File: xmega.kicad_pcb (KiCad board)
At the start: 2 copper layers, 96.5 x 50.8 mm, 93 parts, among them IC1 ATXMEGA128A3U-A, P1 PH_PWR, P3 PH_CURRENT, P5 USB_OTG, P6 PH_TWI, P7 PH_PA, P8 CONN_01X16, Q1 SI2323DS, SW0 TACTB-24R-F, SW1 TACTB-24R-F, SW2 TACTB-24R-F, SW3 TACTB-24R-F, U1 AT45DB161E - EIAJ SOIC, U2 MC78M05CDT, U3 AP1117, U4 LM4040BIM3-2.5, U5 USBLC62, U6 MAX3232EID, U7 micro_sd_card

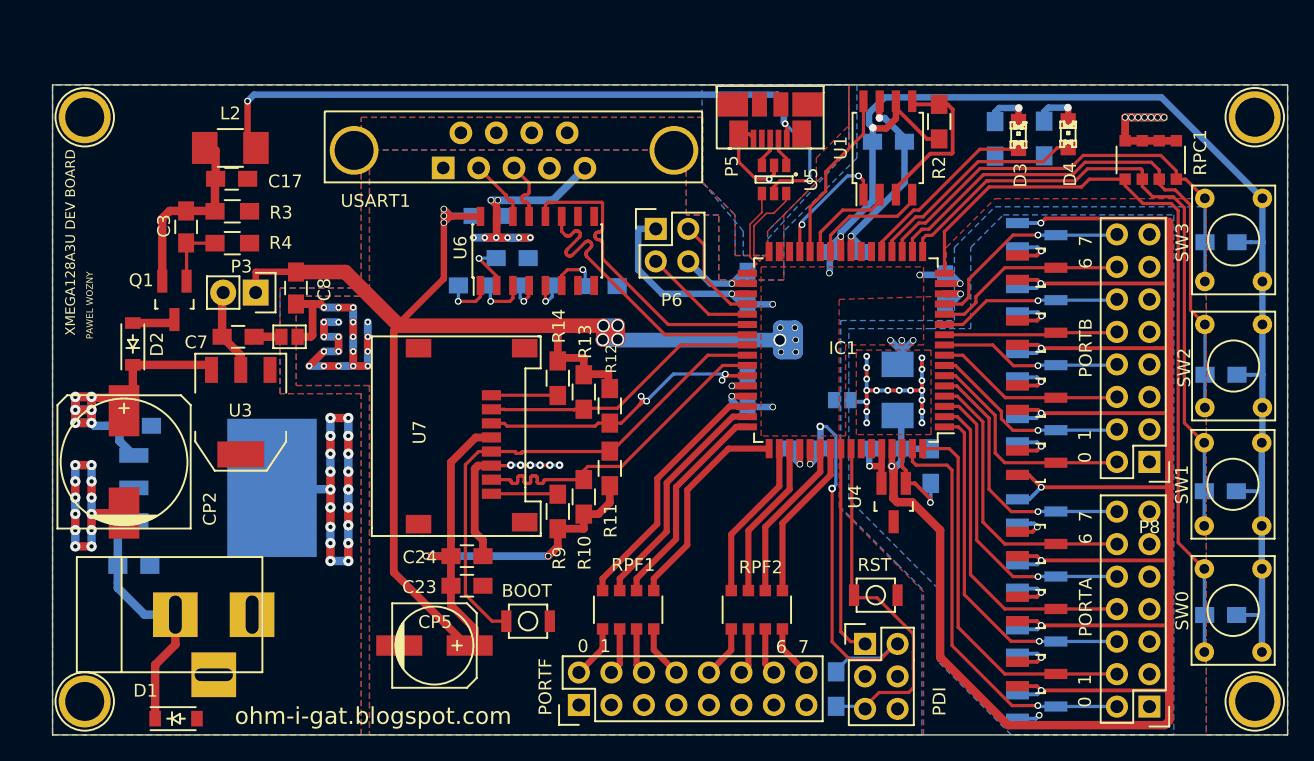
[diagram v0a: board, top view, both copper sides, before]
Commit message: dd
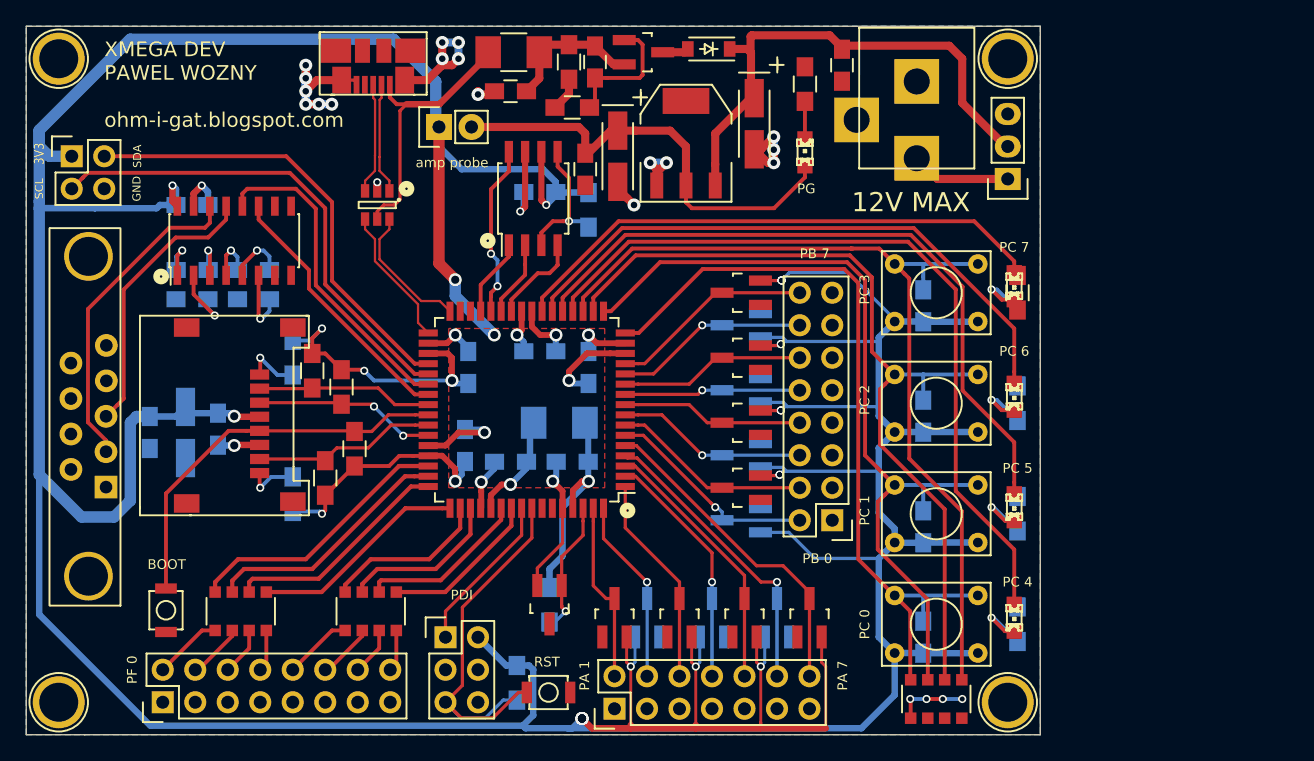
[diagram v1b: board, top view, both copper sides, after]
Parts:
- removed BOOT: boot, woznyLIB:B3U-1000P
- removed C24: 1n, Capacitors_SMD:C_0805_HandSoldering
- removed C25, C26, C27, C28, C4: 100n, Capacitors_SMD:C_0805_HandSoldering
- removed CP2: 100u, Capacitors_SMD:c_elec_10x7.7
- removed CP5: 100u, Capacitors_SMD:c_elec_6.3x5.3
- removed D1: SS14, Diodes_SMD:SOD-123
- removed Digital: PH_DIGITAL IO, Pin_Headers:Pin_Header_Straight_2x08
- removed JP1, JP2: Jumper_NC_Small, Connect:GS2
- removed PDI: PH_PDI, Pin_Headers:Pin_Header_Straight_2x03
- removed R5: 17k8, Resistors_SMD:R_0805_HandSoldering
- removed the REF** at (58.4, 119.3)
- removed the REF** at (58.4, 73.6)
- removed the REF** at (149.8, 119.3)
- removed the REF** at (149.8, 73.6)
- removed RST: rst, woznyLIB:B3U-1000P
- removed SW0: TACTB-24R-F, woznyLIB:B3F-1022
- removed U7: micro_sd_card, woznyLIB:112C-TBAR-R02
- added C19: 100n, Capacitors_SMD:C_0805_HandSoldering, B.Cu at (66.8, 85.6)
- added C20: 100n, Capacitors_SMD:C_0805_HandSoldering, B.Cu at (71.6, 85.6)
- added C21: 100n, Capacitors_SMD:C_0805_HandSoldering, B.Cu at (66.8, 80.5)
- added C22: 100n, Capacitors_SMD:C_0805_HandSoldering, B.Cu at (66.8, 87.9)
- added CT1: 100u, Capacitors_Tantalum_SMD:TantalC_SizeA_EIA-3216_HandSoldering, F.Cu at (110.7, 74.2)
- added CT2: 100u, Capacitors_Tantalum_SMD:TantalC_SizeA_EIA-3216_HandSoldering, F.Cu at (100.1, 76.7)
- added CT3: 100u, Capacitors_Tantalum_SMD:TantalC_SizeA_EIA-3216_HandSoldering, B.Cu at (66.3, 98.3)
- added D21: LED, LEDs:LED-0805, F.Cu at (131.0, 104.1)
- added D22: LED, LEDs:LED-0805, F.Cu at (131.0, 112.8)
- added D5: Dprot, Housings_SOT-23_SOT-143_TSOT-6:SOT-23_Handsoldering, B.Cu at (102.4, 112.8)
- added P2: PH_PDI, Pin_Headers:Pin_Header_Straight_2x03, F.Cu at (86.6, 114.3)
- added P4: PH_DIGITAL IO, Pin_Headers:Pin_Header_Straight_2x08, F.Cu at (64.5, 119.4)
- added R16: 220, Resistors_SMD:R_0805_HandSoldering, B.Cu at (131.3, 104.6)
- added R17: 220, Resistors_SMD:R_0805_HandSoldering, B.Cu at (131.3, 113.3)
- added R6: 220, Resistors_SMD:R_0805_HandSoldering, F.Cu at (114.7, 71.1)
- added R7: 17k8, Resistors_SMD:R_0805_HandSoldering, B.Cu at (94.7, 111.7)
- added REF**: 1pin, Connect:1pin, F.Cu at (56.4, 69.1)
- added REF**: 1pin, Connect:1pin, F.Cu at (130.5, 69.1)
- added REF**: 1pin, Connect:1pin, F.Cu at (56.4, 119.4)
- added REF**: 1pin, Connect:1pin, F.Cu at (130.5, 119.4)
- added SW4: TACTB-24R-F, woznyLIB:SWITCH__B3F-1022, F.Cu at (124.9, 113.3)
- added SW5: TACTB-24R-F, woznyLIB:SWITCH__B3F-1022, F.Cu at (124.9, 104.6)
- added SW6: TACTB-24R-F, woznyLIB:SWITCH__B3F-1022, F.Cu at (124.9, 96.0)
- added SW7: TACTB-24R-F, woznyLIB:SWITCH__B3F-1022, F.Cu at (124.9, 87.4)
- C1, C12, C2, D10, D12, D14, D16, D18, D6, D8: moved to F.Cu
- C14: value 100n -> 1n
- C17, C23, C7, C8, D11, D13, D15, D17, D7, D9, R13, R2: moved to B.Cu
- D19: value Dprot -> LED; footprint Housings_SOT-23_SOT-143_TSOT-6:SOT-23_Handsoldering -> LEDs:LED-0805
- D20: value Dprot -> LED; footprint Housings_SOT-23_SOT-143_TSOT-6:SOT-23_Handsoldering -> LEDs:LED-0805; moved to F.Cu
- D3: value LED -> PG3.3
- D4: value LED -> Dprot; footprint LEDs:LED-0805 -> Housings_SOT-23_SOT-143_TSOT-6:SOT-23_Handsoldering
- P1: footprint Connect:BARREL_JACK -> woznyLIB:BARREL_JACK
- P5: footprint woznyLIB:G3515-10 -> woznyLIB:uUSB__G3515-10
- P6: value PH_TWI -> PH_PA; footprint Pin_Headers:Pin_Header_Straight_2x02 -> Pin_Headers:Pin_Header_Straight_2x07
- P7: value PH_PA -> CONN_01X16; footprint Pin_Headers:Pin_Header_Straight_2x07 -> Pin_Headers:Pin_Header_Straight_2x08
- P8: value CONN_01X16 -> PH_TWI; footprint Pin_Headers:Pin_Header_Straight_2x08 -> Pin_Headers:Pin_Header_Straight_2x02
- R14: value 50K -> 220
- R8: value 220 -> 50K
- SW1: value TACTB-24R-F -> boot; footprint woznyLIB:B3F-1022 -> woznyLIB:SWITCH__B3U-1000P
- SW2: value TACTB-24R-F -> rst; footprint woznyLIB:B3F-1022 -> woznyLIB:SWITCH__B3U-1000P
- SW3: value TACTB-24R-F -> SPST; footprint woznyLIB:B3F-1022 -> Pin_Headers:Pin_Header_Straight_1x03
- U2: value MC78M05CDT -> AP1117; footprint SMD_Packages:TO-263 -> SMD_Packages:SOT-223; moved to F.Cu
- U3: value AP1117 -> LM4040BIM3-2.5; footprint SMD_Packages:SOT-223 -> Housings_SOT-23_SOT-143_TSOT-6:SOT-23_Handsoldering
- U4: value LM4040BIM3-2.5 -> USBLC62; footprint Housings_SOT-23_SOT-143_TSOT-6:SOT-23_Handsoldering -> Housings_SOT-23_SOT-143_TSOT-6:SOT-23-6
- U5: value USBLC62 -> micro_sd_card; footprint Housings_SOT-23_SOT-143_TSOT-6:SOT-23-6 -> woznyLIB:SDcard__112C-TBAR-R02
- USART1: footprint woznyLIB:DBR09F -> woznyLIB:USART__DBR09F
- moved P8 87.5 mm to (57.4, 76.7), turned to 0 degrees
- moved SW1 84.2 mm to (64.7, 113.9), turned to 90 degrees
- moved P1 71.6 mm to (123.4, 70.7), turned to 270 degrees
- moved R8 61.5 mm to (74.7, 103.1), turned to 90 degrees
- moved SW2 57.8 mm to (96.3, 118.6), turned to 180 degrees
- moved C17 57.1 mm to (123.9, 97.0), turned to 90 degrees
- moved C13 56.2 mm to (63.5, 98.3), turned to 270 degrees
- moved D4 51.8 mm to (99.8, 112.8), turned to 0 degrees
- moved U2 50.9 mm to (105.4, 75.7), turned to 0 degrees
- moved D2 50.6 mm to (107.2, 68.3), turned to 180 degrees
- moved U5 46.8 mm to (69.1, 96.5)
- moved U4 46.6 mm to (81.3, 80.5), turned to 270 degrees
- moved C14 45.9 mm to (68.8, 98.0), turned to 270 degrees
- moved RPC1 45.3 mm to (124.9, 119.1)
- moved Q1 41.5 mm to (102.1, 68.6), turned to 270 degrees
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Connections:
- C1 pad 1: Net-(C1-Pad1) -> +5V
- C10 pad 2: GNDD -> GND
- C11 pad 1: +3V3 -> +3.3VADC
- C11 pad 2: GNDD -> GND
- C12 pad 1: +3V3 -> +5V
- C12 pad 2: GNDD -> GND
- C13 pad 2: GNDD -> GND
- C14 pad 2: GNDD -> GND
- C15 pad 2: GNDD -> /buttons/O0
- C16 pad 1: +3.3VADC -> +3V3
- C16 pad 2: GNDA -> /buttons/O1
- C17 pad 1: +5V -> +3V3
- C17 pad 2: GND -> /buttons/O2
- C18 pad 1: GNDD -> +3V3
- C18 pad 2: Net-(C18-Pad2) -> /buttons/O3
- C2 pad 2: Net-(C2-Pad2) -> GND
- C23 pad 1: +3V3 -> GND
- C23 pad 2: GNDD -> Net-(C23-Pad2)
- C3 pad 1: +5V -> /Vcc_5_3V/CC0
- C3 pad 2: Net-(C3-Pad2) -> GND
- C5 pad 1: /Vcc_5_3V/5VUSB -> +3V3
- C6 pad 1: GNDD -> +3V3
- C6 pad 2: +3V3 -> GND
- C7 pad 1: /Vcc_5_3V/CC0 -> +3V3
- C8 pad 2: GNDD -> GND
- C9 pad 1: GNDD -> +3V3
- C9 pad 2: Net-(C9-Pad2) -> GND
- D10 pad 1: GNDA -> GND
- D10 pad 2: +3.3VADC -> +3V3
- D10 pad 3: /Dpa/IO5 -> /Dpa/IO7
- D11 pad 1: GNDA -> GND
- D11 pad 2: +3.3VADC -> +3V3
- D11 pad 3: /Dpa/IO6 -> /Dpb/IO0
- D12 pad 1: GNDA -> GND
- D12 pad 2: +3.3VADC -> +3V3
- D12 pad 3: /Dpa/IO7 -> /Dpb/IO1
- D13 pad 1: GNDA -> GND
- D13 pad 2: +3.3VADC -> +3V3
- D13 pad 3: /Dpb/IO0 -> /Dpb/IO2
- D14 pad 1: GNDA -> GND
- D14 pad 2: +3.3VADC -> +3V3
- D14 pad 3: /Dpb/IO1 -> /Dpb/IO3
- D15 pad 1: GNDA -> GND
- D15 pad 2: +3.3VADC -> +3V3
- D15 pad 3: /Dpb/IO2 -> /Dpb/IO4
- D16 pad 1: GNDA -> GND
- D16 pad 2: +3.3VADC -> +3V3
- D16 pad 3: /Dpb/IO3 -> /Dpb/IO5
- D17 pad 1: GNDA -> GND
- D17 pad 2: +3.3VADC -> +3V3
- D17 pad 3: /Dpb/IO4 -> /Dpb/IO6
- D18 pad 1: GNDA -> GND
- D18 pad 2: +3.3VADC -> +3V3
- D18 pad 3: /Dpb/IO5 -> /Dpb/IO7
- D19 pad 1: GNDA -> Net-(D19-Pad1)
- D19 pad 2: +3.3VADC -> /diode/diode3
- D2 pad 1: /Vcc_5_3V/5VUSB -> Net-(C2-Pad1)
- D20 pad 1: GNDA -> Net-(D20-Pad1)
- D20 pad 2: +3.3VADC -> /diode/diode2
- D3 pad 2: /diode/diode1 -> /Vcc_5_3V/CC0
- D4 pad 1: Net-(D4-Pad1) -> GND
- D4 pad 2: /diode/diode0 -> +3V3
- D6 pad 1: GNDA -> GND
- D6 pad 2: +3.3VADC -> +3V3
- D6 pad 3: /Dpa/IO1 -> /Dpa/IO3
- D7 pad 1: GNDA -> GND
- D7 pad 2: +3.3VADC -> +3V3
- D7 pad 3: /Dpa/IO2 -> /Dpa/IO4
- D8 pad 1: GNDA -> GND
- D8 pad 2: +3.3VADC -> +3V3
- D8 pad 3: /Dpa/IO3 -> /Dpa/IO5
- D9 pad 1: GNDA -> GND
- D9 pad 2: +3.3VADC -> +3V3
- D9 pad 3: /Dpa/IO4 -> /Dpa/IO6
- IC1 pad 14: GNDD -> GND
- IC1 pad 22: (no net) -> /diode/diode2
- IC1 pad 23: (no net) -> /diode/diode3
- IC1 pad 24: GNDD -> GND
- IC1 pad 34: GNDD -> GND
- IC1 pad 44: GNDD -> GND
- IC1 pad 52: GNDD -> GND
- IC1 pad 60: GNDA -> GND
- P1 pad 1: GND -> /Vcc_5_3V/PWR+
- P1 pad 2: /Vcc_5_3V/PWR+ -> (no net)
- P1 pad 3: (no net) -> GND
- P6 pad 1: +3V3 -> GND
- P6 pad 2: /twi/SDA -> /Dpa/IO1
- P6 pad 3: /twi/SCL -> GND
- P6 pad 4: GNDD -> /Dpa/IO2
- P7 pad 1: GNDA -> GND
- P7 pad 10: /Dpa/IO5 -> /Dpb/IO4
- P7 pad 11: GNDA -> GND
- P7 pad 12: /Dpa/IO6 -> /Dpb/IO5
- P7 pad 13: GNDA -> GND
- P7 pad 14: /Dpa/IO7 -> /Dpb/IO6
- P7 pad 2: /Dpa/IO1 -> /Dpb/IO0
- P7 pad 3: GNDA -> GND
- P7 pad 4: /Dpa/IO2 -> /Dpb/IO1
- P7 pad 5: GNDA -> GND
- P7 pad 6: /Dpa/IO3 -> /Dpb/IO2
- P7 pad 7: GNDA -> GND
- P7 pad 8: /Dpa/IO4 -> /Dpb/IO3
- P7 pad 9: GNDA -> GND
- P8 pad 1: GNDA -> +3V3
- P8 pad 2: /Dpb/IO0 -> /twi/SDA
- P8 pad 3: GNDA -> /twi/SCL
- P8 pad 4: /Dpb/IO1 -> GND
- Q1 pad 1: Net-(C3-Pad2) -> Net-(C1-Pad2)
- R10 pad 2: /SD_CARD/MISO -> /SD_CARD/SCK
- R11 pad 2: /SD_CARD/SCK -> /SD_CARD/MOSI
- R12 pad 2: /SD_CARD/MOSI -> /SD_CARD/~SS
- R13 pad 2: /SD_CARD/~SS -> Net-(R13-Pad2)
- R14 pad 1: +3V3 -> Net-(D19-Pad1)
- R14 pad 2: Net-(R14-Pad2) -> GND
- R15 pad 1: Net-(D4-Pad1) -> Net-(D20-Pad1)
- R15 pad 2: GNDD -> GND
- R4 pad 1: Net-(C3-Pad2) -> Net-(C1-Pad2)
- R8 pad 1: Net-(D3-Pad1) -> +3V3
- R8 pad 2: GNDD -> Net-(R8-Pad2)
- R9 pad 2: Net-(R9-Pad2) -> /SD_CARD/MISO
- RPC1 pad 1: GNDD -> /buttons/O3
- RPC1 pad 2: GNDD -> /buttons/O2
- RPC1 pad 3: GNDD -> /buttons/O1
- RPC1 pad 4: GNDD -> /buttons/O0
- RPC1 pad 5: /buttons/O0 -> GND
- RPC1 pad 6: /buttons/O1 -> GND
- RPC1 pad 7: /buttons/O2 -> GND
- RPC1 pad 8: /buttons/O3 -> GND
- SW1 pad 1: /buttons/O1 -> GND
- SW1 pad 2: +3V3 -> /SD_CARD/SCK
- SW2 pad 1: /buttons/O2 -> GND
- SW2 pad 2: +3V3 -> PDI_CLK
- SW3 pad 1: /buttons/O3 -> /Vcc_5_3V/PWR+
- SW3 pad 2: +3V3 -> Net-(C2-Pad1)
- U1 pad 7: GNDD -> GND
- U2 pad 1: /Vcc_5_3V/PWR+ -> GND
- U2 pad 2: GND -> /Vcc_5_3V/CC0
- U2 pad 3: /Vcc_5_3V/5VUSB -> Net-(C2-Pad1)
- U3 pad 1: GND -> /vrefA/Vref
- U3 pad 2: /Vcc_5_3V/CC0 -> GND
- U3 pad 3: /Vcc_5_3V/5VUSB -> (no net)
- U4 pad 1: /vrefA/Vref -> /USB/D1-
- U4 pad 2: GNDA -> GND
- U4 pad 3: (no net) -> /USB/D1+
- U5 pad 1: /USB/D1- -> Net-(R13-Pad2)
- U5 pad 2: GND -> /SD_CARD/~SS
- U5 pad 3: /USB/D1+ -> /SD_CARD/MOSI
- U5 pad 4: /USB/D2+ -> +3V3
- U5 pad 5: Net-(L2-Pad2) -> /SD_CARD/SCK
- U5 pad 6: /USB/D2- -> GND
- U6 pad 1: Net-(C1-Pad1) -> Net-(C19-Pad1)
- U6 pad 15: GNDD -> GND
- U6 pad 2: Net-(C9-Pad2) -> Net-(C22-Pad2)
- U6 pad 3: Net-(C1-Pad2) -> Net-(C19-Pad2)
- U6 pad 4: Net-(C2-Pad1) -> Net-(C20-Pad1)
- U6 pad 5: Net-(C2-Pad2) -> Net-(C20-Pad2)
- U6 pad 6: Net-(C18-Pad2) -> Net-(C23-Pad2)
- USART1 pad 5: GNDD -> GND
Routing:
- net +3.3VADC: track 195.6 -> 17.2 mm, vias 9 -> 1
- net +3V3: track 320.9 -> 471.9 mm, vias 30 -> 29
- net GNDD: track 110.4 -> 0.00 mm, vias 47 -> 0
- net GNDA: track 50.4 -> 0.00 mm, vias 27 -> 0
- net /diode/diode2: track 0.00 -> 46.9 mm
- net /diode/diode0: track 17.6 -> 60.8 mm
- net /diode/diode3: track 0.00 -> 42.6 mm
- net /diode/diode1: track 14.5 -> 53.9 mm
- net /Vcc_5_3V/5VUSB: track 38.6 -> 0.00 mm, vias 6 -> 0
- net Net-(C2-Pad1): track 2.77 -> 41.0 mm, vias 1 -> 0
- net Net-(L2-Pad2): track 58.2 -> 21.1 mm, vias 3 -> 0
- net /buttons/O3: track 35.6 -> 70.9 mm
- net GND: track 60.3 -> 94.5 mm
- net /twi/SCL: track 8.87 -> 38.7 mm
- net /Vcc_5_3V/CC0: track 6.78 -> 35.5 mm
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- removed copper zone on B.Cu, net GNDA
- removed copper zone on F.Cu, net GNDA
- removed copper zone on B.Cu, net GNDD
- removed copper zone on F.Cu, net GNDD
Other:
- board size 96.5 x 50.8 mm -> 79.2 x 55.4 mm
- net class Default: trace_width 0.254 -> 0.3048; via_dia 0.5334 -> 0.635; via_drill 0.3302 -> 0.381
- net class GNDA removed
- net class GNDD removed
- net class IO_DIGITAL removed
- net class PDI removed
- net class PWR added: clearance 0.381, trace_width 0.635, via_dia 1.016, via_drill 0.508
- net class PWR3.3: clearance 0.254 -> 0.2286; trace_width 0.6604 -> 0.508; via_dia 0.8128 -> 1.016; via_drill 0.6096 -> 0.635
- rule trace_min: 3.87096 -> 0.1524
- rule via_min_size: 12.9032 -> 0.508
- board text added: "12V MAX"
- board text added: "3V3"
- board text added: "BOOT"
- board text added: "GND"
- board text added: "PA 1"
- board text added: "PA 7"
- board text added: "PB 0"
- board text added: "PB 7"
- board text added: "PC 0"
- board text added: "PC 1"
- board text added: "PC 2"
- board text added: "PC 3"
- board text added: "PC 4"
- board text added: "PC 5"
- board text added: "PC 6"
- board text added: "PC 7"
- board text added: "PDI"
- board text added: "PF 0"
- board text added: "PG"
- board text added: "RST"
- board text added: "SCL"
- board text added: "SDA"
- board text added: "XMEGA DEV PAWEL WOZNY ohm-i-gat.blogspot.com"
- board text added: "amp probe"
- board text added: "r1_150730"
- board text removed: "0 1"
- board text removed: "6 7"
- board text removed: "PAWEL WOZNY"
- board text removed: "PORTA"
- board text removed: "PORTB"
- board text removed: "PORTF"
- board text removed: "XMEGA128A3U DEV BOARD"
- board text removed: "ohm-i-gat.blogspot.com"
